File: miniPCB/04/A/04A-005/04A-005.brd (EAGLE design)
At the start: 24 parts

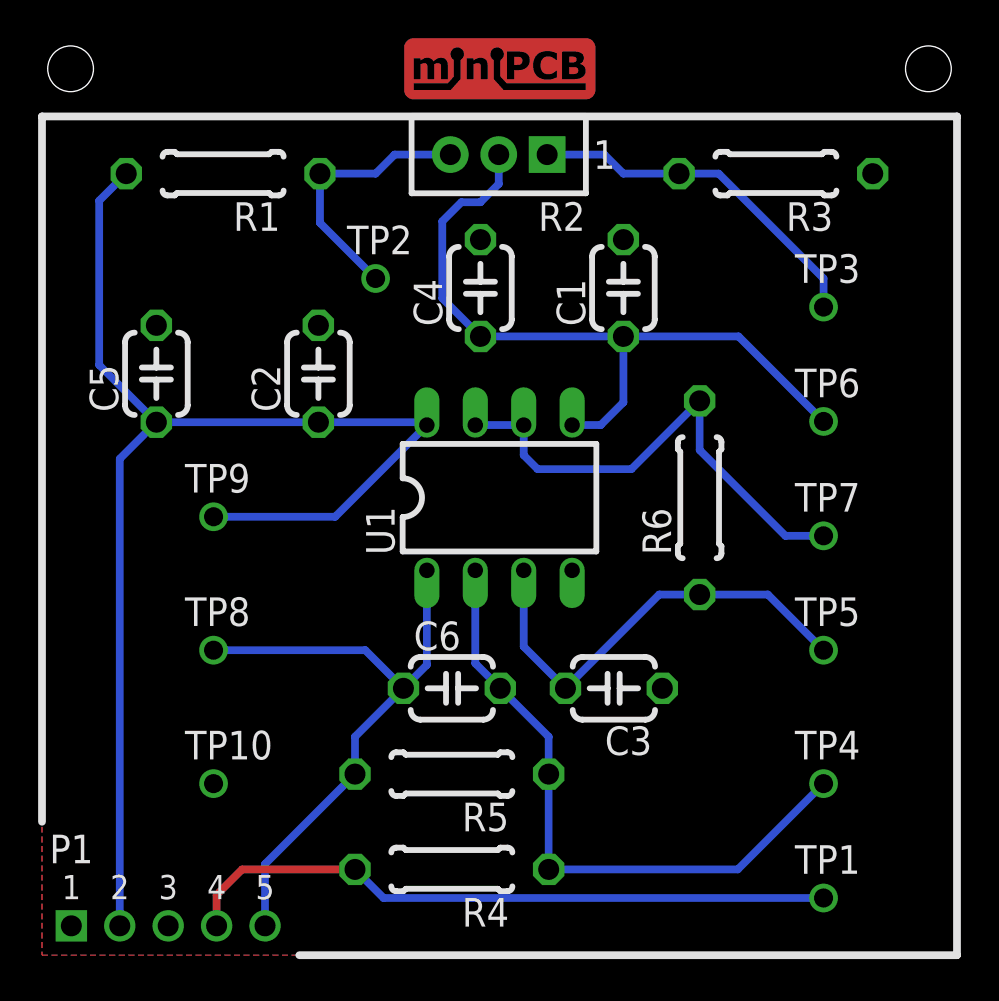
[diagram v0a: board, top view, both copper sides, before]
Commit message: NM.14JAN2023
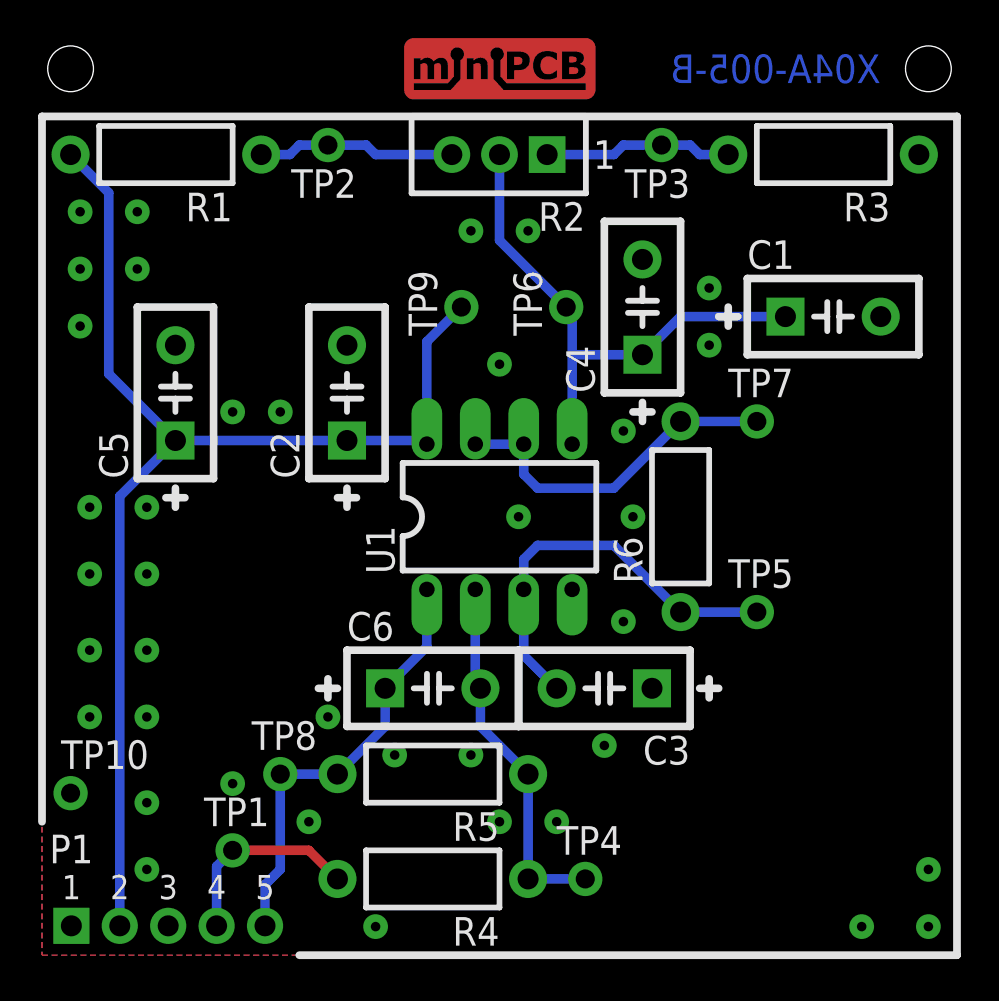
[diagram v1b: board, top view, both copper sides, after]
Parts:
- moved TP1 31.1 mm to (11.0, 6.50)
- moved TP9 17.0 mm to (23.0, 35.0), turned to 90 degrees
- moved TP6 14.8 mm to (28.5, 35.0), turned to 90 degrees
- moved TP4 13.5 mm to (29.5, 5.00)
- moved TP3 12.0 mm to (33.5, 43.5), turned to 180 degrees
- moved C1 11.1 mm to (42.5, 34.5), turned to 0 degrees
- moved C4 8.56 mm to (32.5, 35.0)
- moved TP10 7.52 mm to (2.50, 9.50)
- moved TP2 7.43 mm to (16.0, 43.5), turned to 180 degrees
- moved TP8 7.38 mm to (13.5, 10.5)
- moved TP7 6.95 mm to (38.5, 29.0)
- moved TP5 4.03 mm to (38.5, 19.0)
- moved R1 3.16 mm to (7.50, 43.0)
- moved R3 2.69 mm to (42.0, 43.0)
- moved C2 1.80 mm to (17.0, 30.5)
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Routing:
- net IN: track 34.6 -> 10.4 mm
- net VFB: track 33.6 -> 19.3 mm
- net OUT: track 33.0 -> 22.9 mm
- net N$1: track 38.7 -> 28.8 mm
- net P1.1: track 18.7 -> 9.91 mm
- net VREF: track 26.1 -> 18.1 mm
- net V+: track 69.6 -> 65.2 mm
- net P1.3: track 14.0 -> 10.4 mm
- net N$2: track 23.9 -> 21.5 mm
